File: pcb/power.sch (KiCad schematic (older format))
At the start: 7 parts, among them U6 ADP2108AUJ-3.3

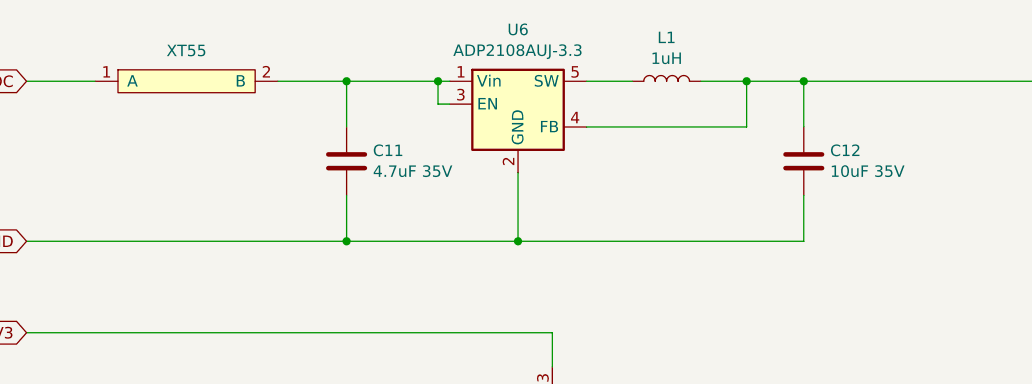
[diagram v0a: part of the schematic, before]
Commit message: Buffers power scheme rework in progress, re-annotate board
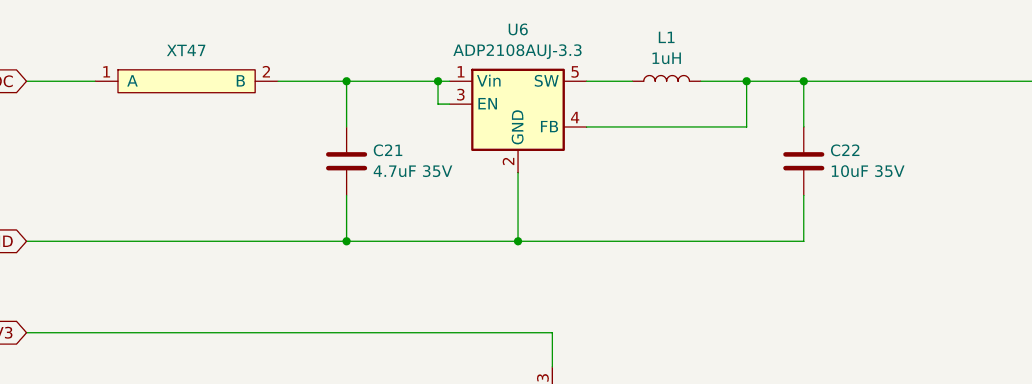
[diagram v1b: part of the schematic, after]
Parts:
- renumbered C11 to C21, C12 to C22, XT55 to XT47
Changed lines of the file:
@@
 $EndComp
 $Comp
-L WM1200:testpoint_cutline XT55
+L WM1200:testpoint_cutline XT47
 U 1 1 5E716612
 P 2300 2050
-F 0 "XT55" H 2300 2233 50  0000 C CNN
+F 0 "XT47" H 2300 2233 50  0000 C CNN
 F 1 "testpoint_cutline" H 2300 2200 50  0001 C CNN
 F 2 "WM1200:testpoint_cutline" H 2450 2050 50  0001 C CNN
@@
 	3400 2000 3450 2000
 $Comp
-L Device:C C11
+L Device:C C21
 U 1 1 5E718DCB
 P 3000 2350
-F 0 "C11" H 3115 2396 50  0000 L CNN
+F 0 "C21" H 3115 2396 50  0000 L CNN
 F 1 "4.7uF 35V" H 3115 2305 50  0000 L CNN
 F 2 "Capacitor_SMD:C_1210_3225Metric_Pad1.42x2.65mm_HandSolder" H 3038 2200 50  0001 C CNN
@@
 	3000 2000 3400 2000
 $Comp
-L Device:C C12
+L Device:C C22
 U 1 1 5E71F97C
 P 5000 2350
-F 0 "C12" H 5115 2396 50  0000 L CNN
+F 0 "C22" H 5115 2396 50  0000 L CNN
 F 1 "10uF 35V" H 5115 2305 50  0000 L CNN
 F 2 "Capacitor_SMD:C_1210_3225Metric_Pad1.42x2.65mm_HandSolder" H 5038 2200 50  0001 C CNN

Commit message: still working
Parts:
- XT47: footprint WM1200:testpoint_cutline -> WM1200:testpoint_cutline_fat
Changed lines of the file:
@@
 F 0 "XT47" H 2300 2233 50  0000 C CNN
 F 1 "testpoint_cutline" H 2300 2200 50  0001 C CNN
-F 2 "WM1200:testpoint_cutline" H 2450 2050 50  0001 C CNN
+F 2 "WM1200:testpoint_cutline_fat" H 2450 2050 50  0001 C CNN
 F 3 "" H 2450 2050 50  0001 C CNN
 	1    2300 2050

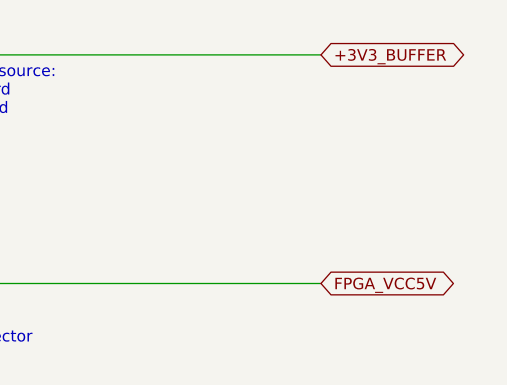
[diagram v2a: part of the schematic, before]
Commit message: Some more work done
I'm too lazy to think about commit messages in my pet project, really
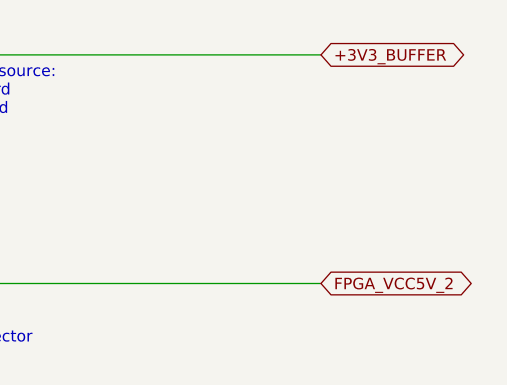
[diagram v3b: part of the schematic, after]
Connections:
- net FPGA_VCC5V renamed FPGA_VCC5V_2
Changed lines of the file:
@@
 +3V3_BUFFER
 Text GLabel 6400 4500 2    50   BiDi ~ 0
-FPGA_VCC5V
+FPGA_VCC5V_2
 $EndSCHEMATC
